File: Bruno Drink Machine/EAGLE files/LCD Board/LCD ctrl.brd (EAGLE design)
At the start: 88.2 x 81.2 mm, 38 parts, among them IC1 PIC24FJ256DA210-I/PT, IC2 IS62LV256AL, IC3 IS62LV256AL, IC4 BA3259H-HRP5, P1 CONN-40P-62684-401100ALF, P18 CONN-8P-PND, P2 USB-CON690-005-299-043

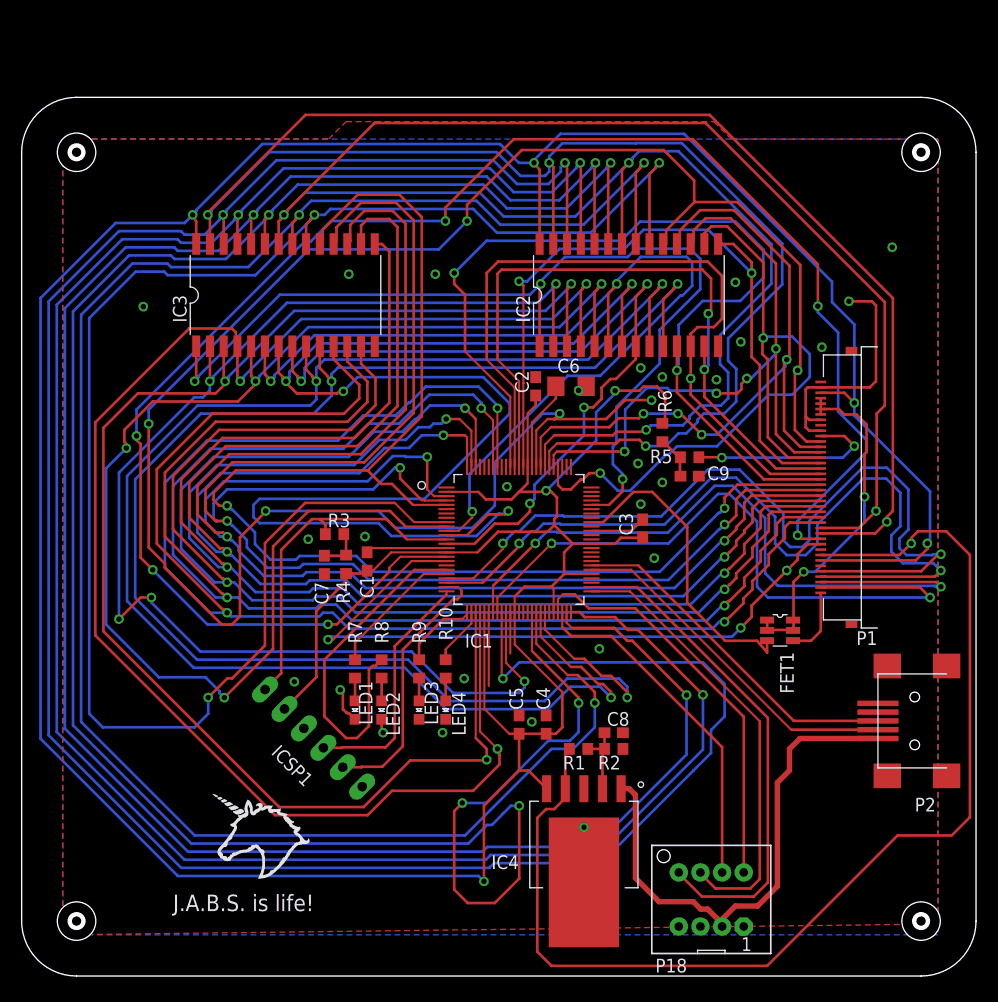
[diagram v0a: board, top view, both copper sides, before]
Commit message: made some of the changes; not all (will need to go through change list and confirm later)
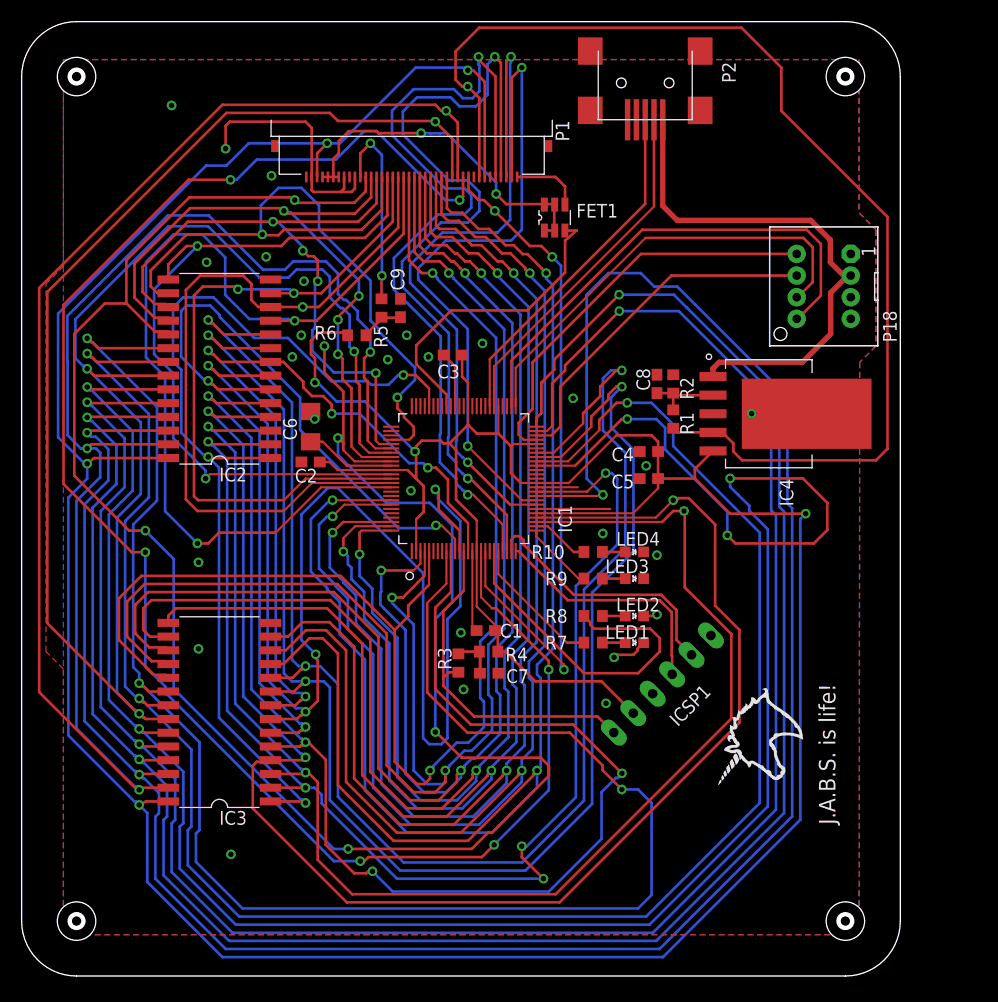
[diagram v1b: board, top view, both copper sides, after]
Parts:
- moved U$32 78.4 mm to (5.08, 83.2), turned to 90 degrees
- moved U$35 78.4 mm to (76.2, 83.2), turned to 90 degrees
- moved U$33 71.1 mm to (5.08, 5.08), turned to 90 degrees
- moved U$34 71.1 mm to (76.2, 5.08), turned to 90 degrees
- moved P2 67.9 mm to (57.7, 85.5), turned to 180 degrees
- moved U$36 61.8 mm to (75.2, 14.0), turned to 90 degrees
- moved P18 57.6 mm to (74.2, 63.8), turned to 90 degrees
- moved P1 51.0 mm to (36.1, 76.4), turned to 180 degrees
- moved U$20 47.1 mm to (68.2, 22.0), turned to 90 degrees
- moved FET1 43.5 mm to (49.3, 70.1), turned to 0 degrees
- moved IC4 43.3 mm to (69.1, 52.0), turned to 270 degrees
- moved IC3 39.0 mm to (18.3, 24.4), turned to 180 degrees
- moved IC2 38.5 mm to (18.3, 56.1), turned to 180 degrees
- moved R2 34.2 mm to (60.2, 54.8), turned to 270 degrees
- moved ICSP1 32.6 mm to (59.2, 27.0), turned to 45 degrees
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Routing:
- net N$6: track 7.28 -> 6.56 mm
- net PGC: track 24.8 -> 24.2 mm
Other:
- board size 88.2 x 81.2 mm -> 81.2 x 88.2 mm
